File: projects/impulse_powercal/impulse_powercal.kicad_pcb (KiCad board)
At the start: 2 copper layers, 40 x 44.2 mm, 12 parts, among them J1 Conn_Coaxial, J2 Conn_01x02_Pin, J3 Conn_01x01_Pin, J4 Conn_01x01_Pin

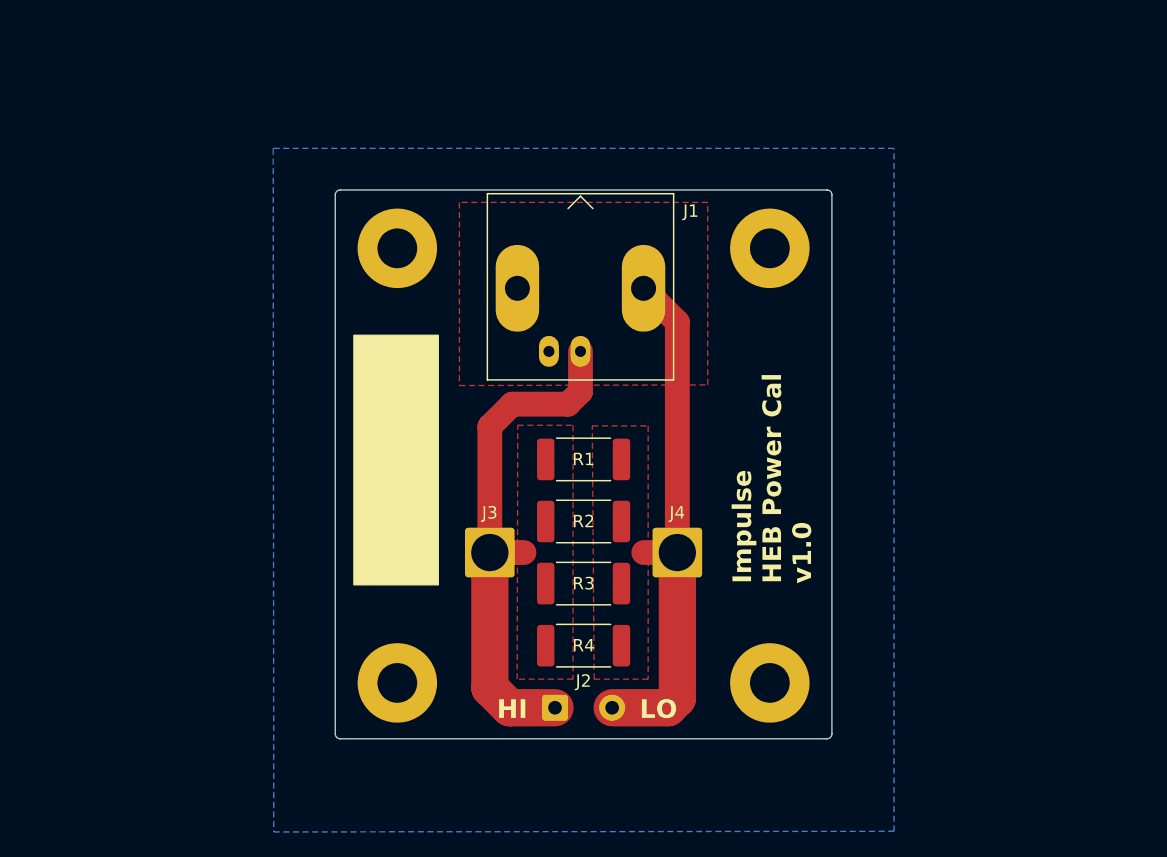
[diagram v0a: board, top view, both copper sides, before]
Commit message: .
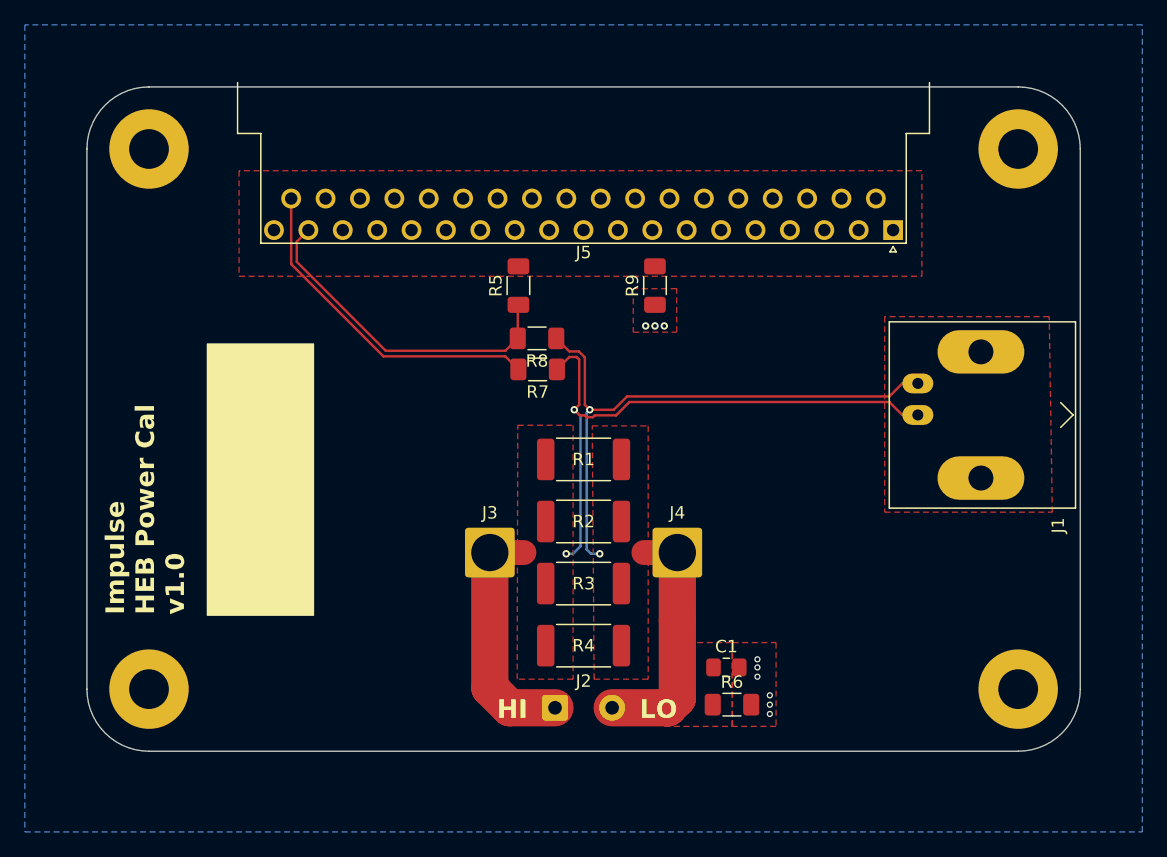
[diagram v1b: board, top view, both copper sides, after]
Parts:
- added C1: DNP, Capacitor_SMD:C_0805_2012Metric_Pad1.18x1.45mm_HandSolder, F.Cu at (111.5, 106.8)
- added J5: DC37_Plug, Connector_Dsub:DSUB-37_Male_Horizontal_P2.77x2.54mm_EdgePinOffset9.40mm, F.Cu at (124.9, 71.5)
- added R5: 100K, Resistor_SMD:R_1206_3216Metric_Pad1.30x1.75mm_HandSolder, F.Cu at (94.8, 76.0)
- added R6: DNP, Resistor_SMD:R_1206_3216Metric_Pad1.30x1.75mm_HandSolder, F.Cu at (112.0, 109.8)
- added R7: 0, Resistor_SMD:R_1206_3216Metric_Pad1.30x1.75mm_HandSolder, F.Cu at (96.3, 82.8)
- added R8: 0, Resistor_SMD:R_1206_3216Metric_Pad1.30x1.75mm_HandSolder, F.Cu at (96.2, 80.2)
- added R9: 0, Resistor_SMD:R_1206_3216Metric_Pad1.30x1.75mm_HandSolder, F.Cu at (105.8, 76.0)
- moved J1 27.6 mm to (126.9, 86.4), turned to -90 degrees
- moved H1 21.5 mm to (65.0, 65.0)
- moved H3 21.5 mm to (135.0, 65.0)
- moved H2 20.0 mm to (65.0, 108.5)
- moved H4 20.0 mm to (135.0, 108.5)
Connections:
- net /HI renamed /HEAT_P
- net /LO renamed /HEAT_N
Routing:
- net /AIN0/1_P: track 0.00 -> 27.1 mm
- net /AIN0/1_N: track 0.00 -> 26.8 mm
- net /HEAT_P: track 41.4 -> 67.5 mm, vias 0 -> 2
- net /HEAT_N: track 42.4 -> 67.2 mm, vias 0 -> 2
- net GND: vias 0 -> 9
- added copper zone on B.Cu, net GND
- added copper zone on F.Cu, net GND
- added copper zone on F.Cu, net GNDJ
- removed copper zone on B.Cu, net (none)
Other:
- board size 40 x 44.2 mm -> 80 x 53.5 mm
